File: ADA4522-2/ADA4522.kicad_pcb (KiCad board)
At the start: 2 copper layers, 30 parts, among them U1 ADA4522-2

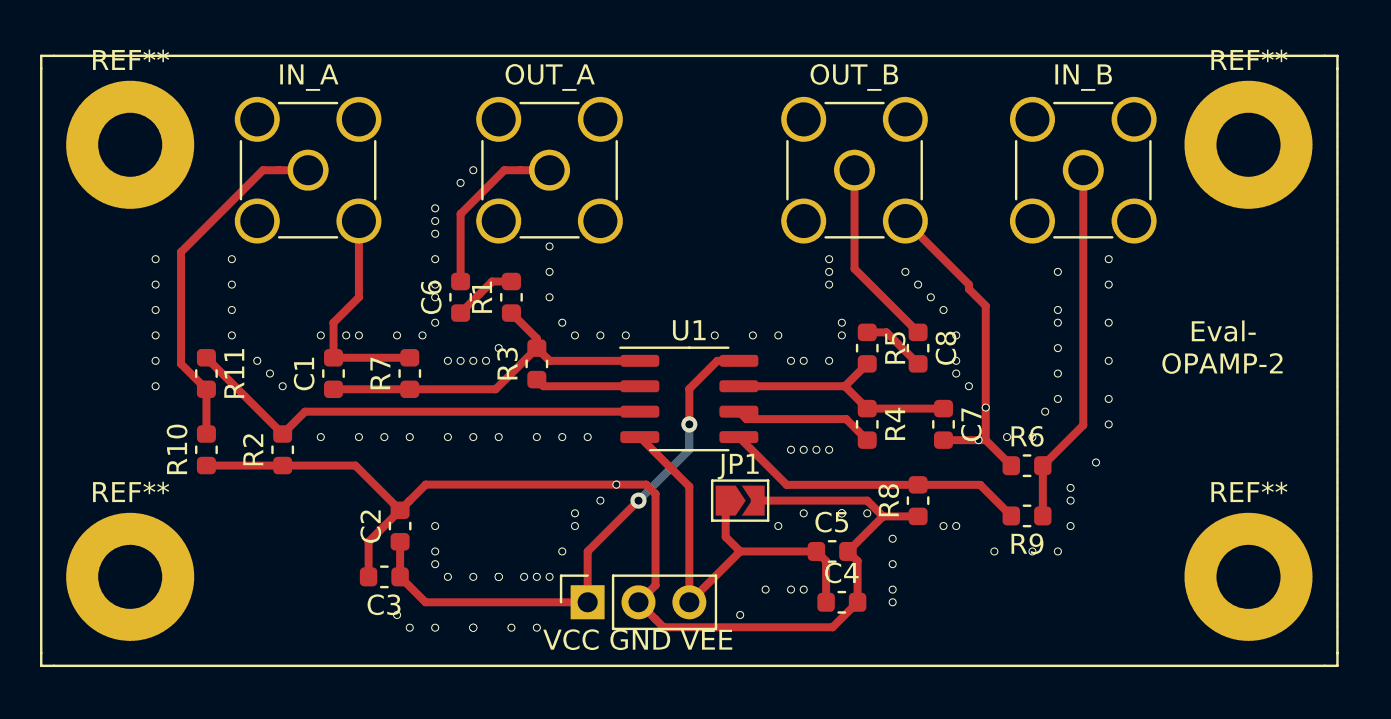
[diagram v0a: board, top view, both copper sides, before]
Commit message: update-version
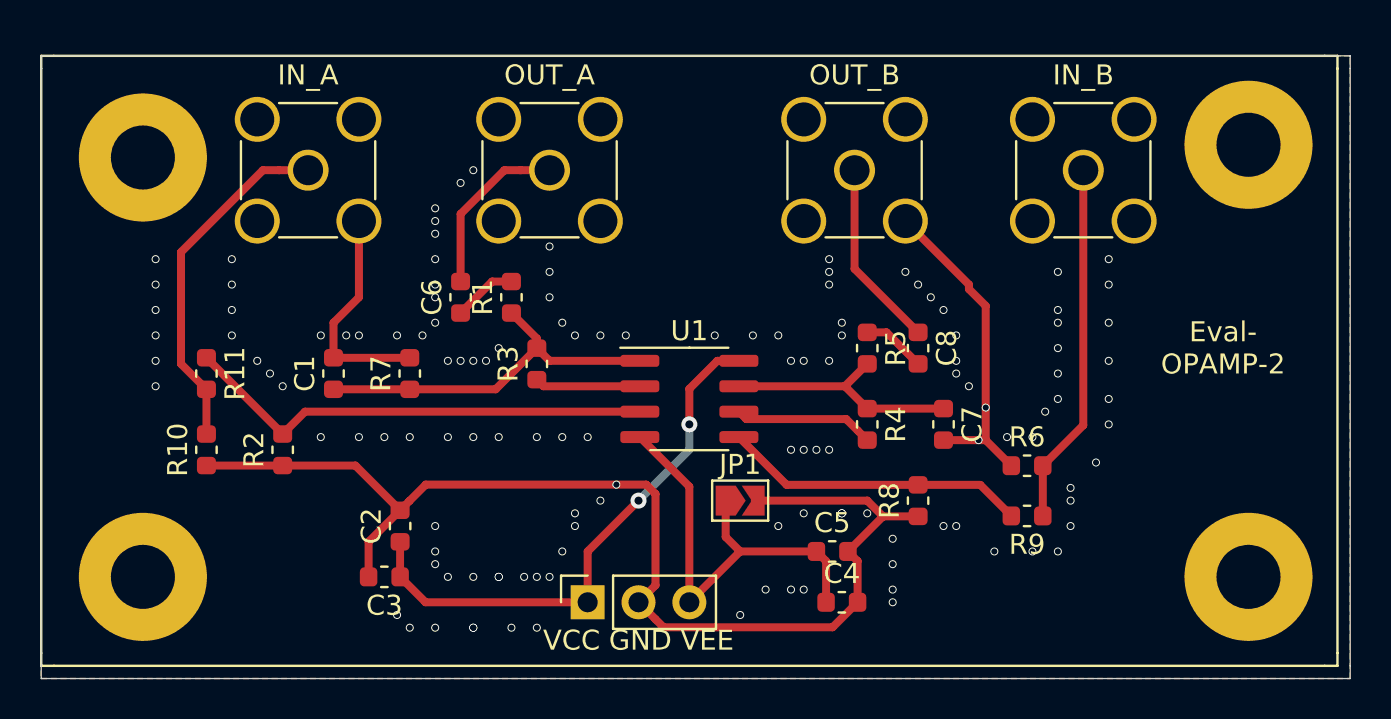
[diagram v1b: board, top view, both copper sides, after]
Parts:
- moved REF** 0.90 mm to (120.0, 71.8)
- moved REF** 0.64 mm to (120.0, 92.7)
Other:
- board outline added: 65.4 x 31.1 mm
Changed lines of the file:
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@@
   (general
     (thickness 1.6)
-    (drawings 13)
+    (drawings 21)
     (tracks 230)
     (zones 0)
@@
     (35 F.Paste user)
     (36 B.SilkS user)
-    (37 F.SilkS user)
+    (37 F.SilkS user hide)
     (38 B.Mask user)
     (39 F.Mask user)
@@
     (tags "mounting hole 3.2mm m3")
     (attr virtual)
-    (fp_text reference REF** (at 0 -4.2) (layer F.SilkS)
+    (fp_text reference REF** (at 0 -4.2) (layer F.SilkS) hide
       (effects (font (size 1 1) (thickness 0.15)))
     )
@@
   )
   (module MountingHole:MountingHole_3.2mm_M3_Pad (layer F.Cu)
-    (at 119.38 92.71)
+    (at 120.015 92.71)
     (descr "Mounting Hole 3.2mm, M3")
     (tags "mounting hole 3.2mm m3")
     (attr virtual)
-    (fp_text reference REF** (at 0 -4.2) (layer F.SilkS)
+    (fp_text reference REF** (at 0 -4.2) (layer F.SilkS) hide
       (effects (font (size 1 1) (thickness 0.15)))
     )
@@
     (tags "mounting hole 3.2mm m3")
     (attr virtual)
-    (fp_text reference REF** (at 0 -4.2) (layer F.SilkS)
+    (fp_text reference REF** (at 0 -4.2) (layer F.SilkS) hide
       (effects (font (size 1 1) (thickness 0.15)))
     )
@@
   )
   (module MountingHole:MountingHole_3.2mm_M3_Pad (layer F.Cu)
-    (at 119.38 71.12)
+    (at 120.015 71.755)
     (descr "Mounting Hole 3.2mm, M3")
     (tags "mounting hole 3.2mm m3")
     (attr virtual)
-    (fp_text reference REF** (at 0 -4.2) (layer F.SilkS)
+    (fp_text reference REF** (at 0 -4.2) (layer F.SilkS) hide
       (effects (font (size 1 1) (thickness 0.15)))
     )
@@
     )
   )
+  (gr_line (start 114.935 97.79) (end 114.935 97.155) (layer Edge.Cuts) (width 0.05))
+  (gr_line (start 180.34 97.155) (end 180.34 97.79) (layer Edge.Cuts) (width 0.05))
+  (gr_line (start 180.34 66.675) (end 180.34 67.31) (layer Edge.Cuts) (width 0.05))
+  (gr_line (start 114.935 67.31) (end 114.935 66.675) (layer Edge.Cuts) (width 0.05))
+  (gr_line (start 180.34 66.675) (end 114.935 66.675) (layer Edge.Cuts) (width 0.05))
+  (gr_line (start 180.34 97.155) (end 180.34 67.31) (layer Edge.Cuts) (width 0.05))
+  (gr_line (start 114.935 97.79) (end 180.34 97.79) (layer Edge.Cuts) (width 0.05))
+  (gr_line (start 114.935 67.31) (end 114.935 97.155) (layer Edge.Cuts) (width 0.05))
   (gr_text "Eval-\nOPAMP-2" (at 173.99 81.28) (layer F.SilkS)
     (effects (font (size 1 1) (thickness 0.15)))
@@
     (polygon
       (pts
-        (xy 114.935 66.675) (xy 114.935 97.155) (xy 179.705 97.155) (xy 179.705 66.675)
+        (xy 114.935 66.675) (xy 114.935 97.79) (xy 180.34 97.79) (xy 180.34 66.675)
       )
     )
@@
     (polygon
       (pts
-        (xy 114.935 66.675) (xy 114.935 97.155) (xy 179.705 97.155) (xy 179.705 66.675)
+        (xy 114.935 66.675) (xy 114.935 97.79) (xy 180.34 97.79) (xy 180.34 66.675)
       )
     )
